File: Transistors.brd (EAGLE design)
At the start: 65 x 55 mm, 68 parts, among them Q1 FDD4141TO252, Q2 FDD4141TO252, Q3 FDD4141TO252, Q4 FDD4141TO252, X1 MSTBA2, X10 22-23-2041, X11 22-23-2041, X12 22-23-2041, X14 22-23-2021, X15 22-23-2021, X16 22-23-2031, X2 22-23-2041, X3 MSTBA2, X4 22-23-2041, X5 MSTBA2, X6 22-23-2041, X7 MSTBA2, X8 22-23-2041, X9 5566-6

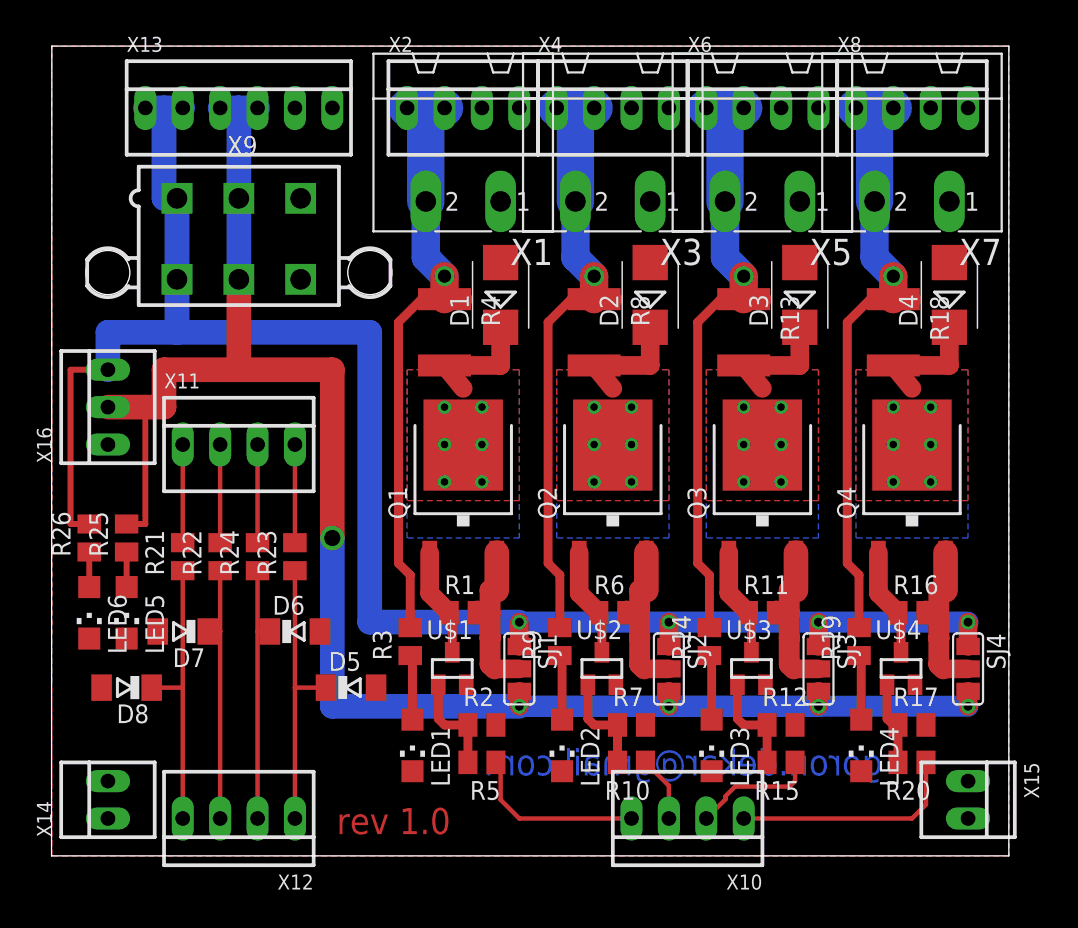
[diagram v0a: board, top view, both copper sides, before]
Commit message: Add values + create compile scheme
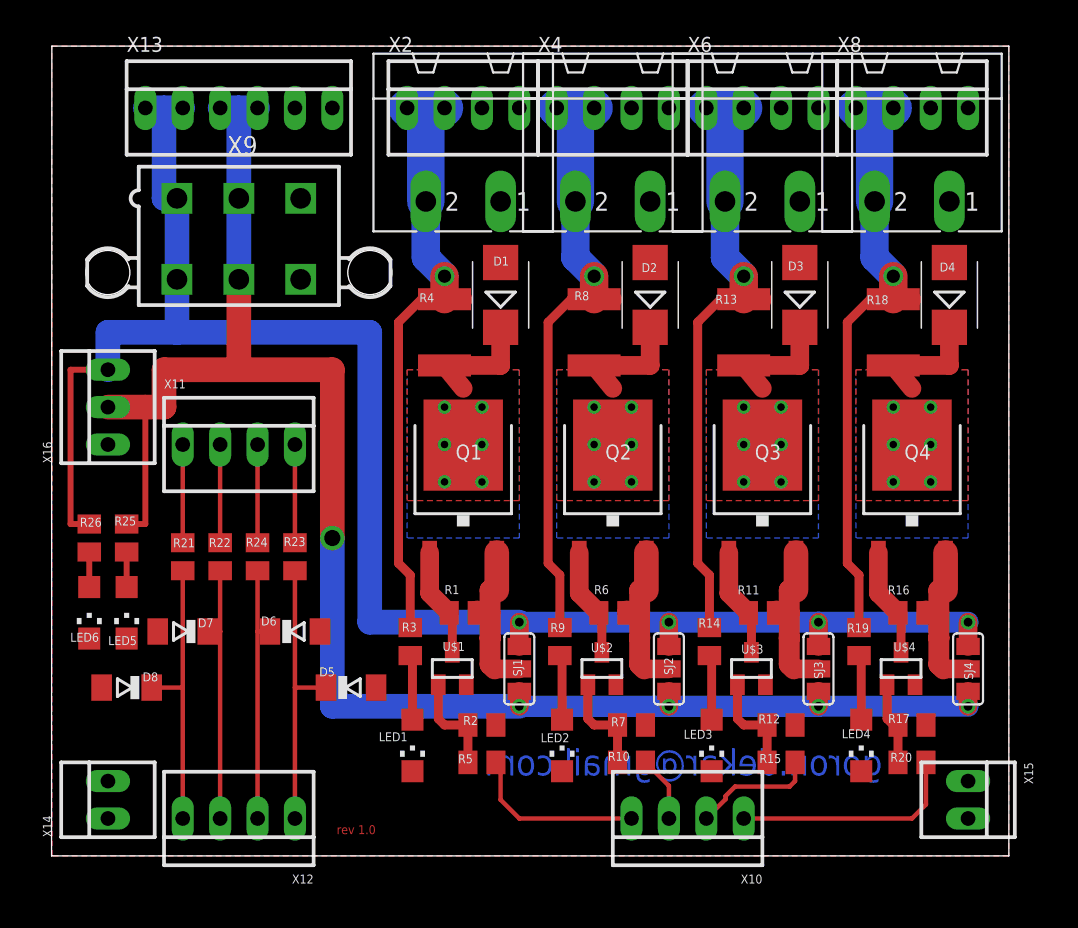
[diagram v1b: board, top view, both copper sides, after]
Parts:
- D5, D6, D7, D8: value (none) -> 3.3
- R1, R11, R16, R26, R6: value (none) -> 510
- R10, R15, R20, R5: value (none) -> 200
- R12, R14, R17, R19, R2, R25, R3, R7, R9: value (none) -> 1000
- R21, R22, R23, R24: value (none) -> 10k
